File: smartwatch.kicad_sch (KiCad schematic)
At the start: 53 parts, among them IC1 W25N01GVZEIG, IC2 NORA-B120-00B, IC3 LM66200DRLR, J1 Charging_Pad-, J2 Charging_Pad+, J3 DS1020-09-15VBT1A, J4 Conn_01x04_Pin, Q1 2N7002, U1 MAX17048G+T10, U11 MCP73831T-2ACI/OT, U2 RV-3028-C7_32.768KHZ_1PPM-TA-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, U3 MAX30102, U4 TPS63001DRCR, U5 CAM-M8C-0, U6 AP7313-18SAG-7, U9 LIS2DE12, X2 9HT10-32.768KBZC-T

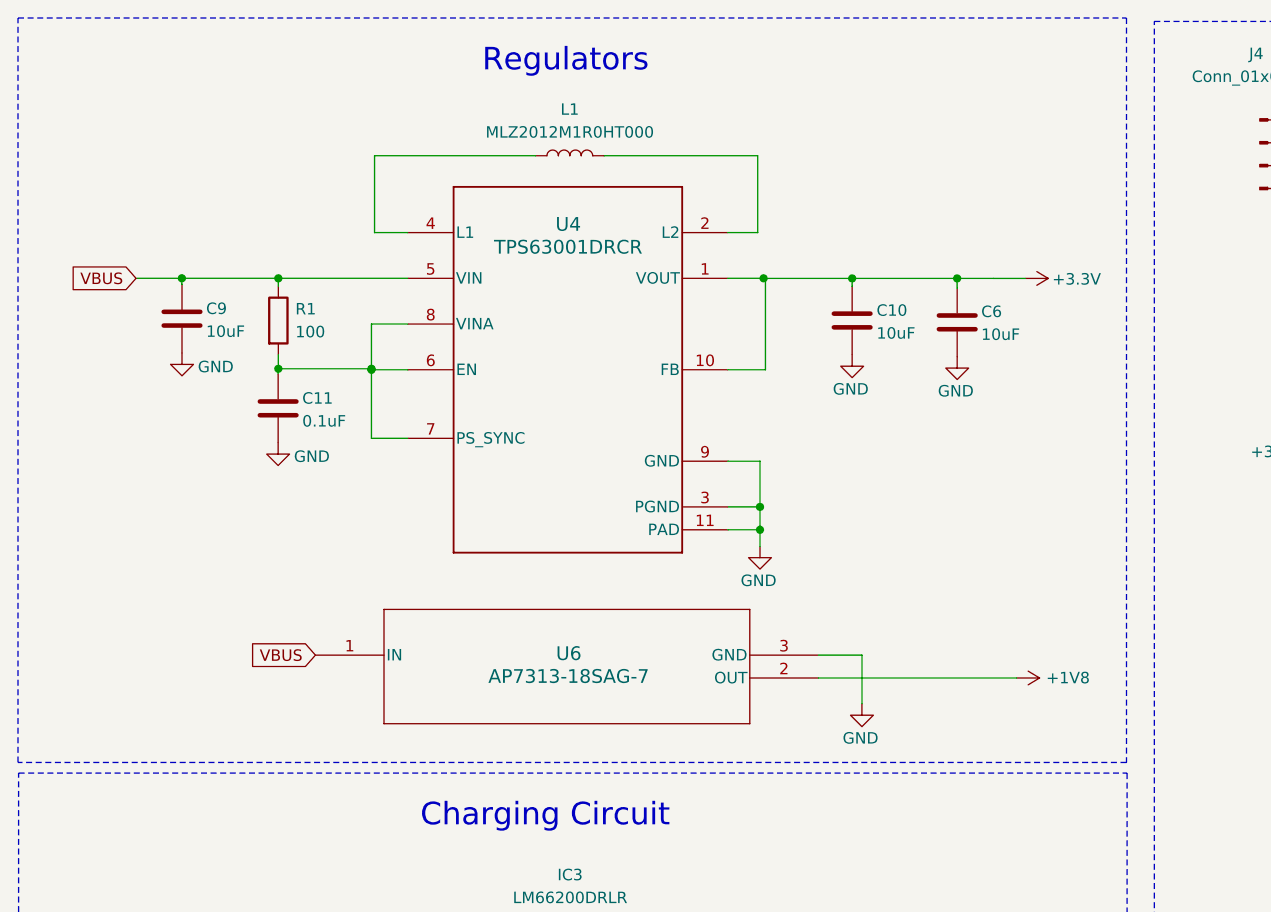
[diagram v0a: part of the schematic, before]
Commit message: update 1
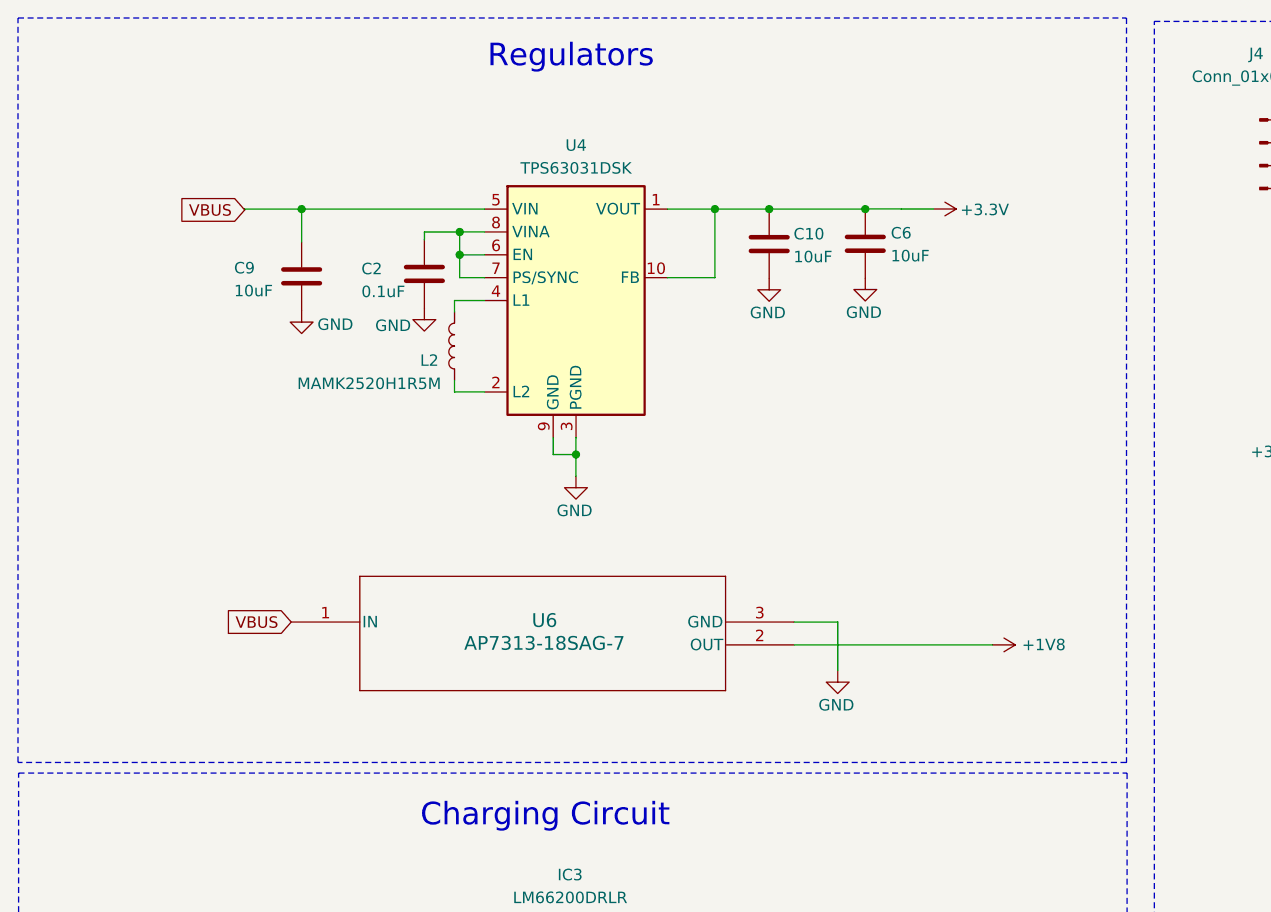
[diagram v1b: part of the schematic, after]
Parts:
- removed C11: 0.1uF, Capacitor_SMD:C_0402_1005Metric, symbol Device:C
- removed L1: MLZ2012M1R0HT000, Inductor_SMD:L_0805_2012Metric, symbol Device:L
- removed R1: 100, Resistor_SMD:R_0402_1005Metric, symbol Device:R
- removed U4: TPS63001DRCR, DRC0010J, symbol TPS63001DRCR:TPS63001DRCR
- added C2: 0.1uF, Capacitor_SMD:C_0402_1005Metric, symbol Device:C
- added L2: MAMK2520H1R5M, Inductor_SMD:L_1008_2520Metric, symbol Device:L
- added U4: TPS63031DSK, Package_SON:WSON-10-1EP_2.5x2.5mm_P0.5mm_EP1.2x2mm, symbol Regulator_Switching:TPS63031DSK
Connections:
- net +3.3V: now also U4.1 (VOUT), U4.10 (FB)
- net GND: now also C2.2, U4.11 (PGND), U4.3 (PGND), U4.9 (GND)
- net VBUS: now also U4.5 (VIN)
- new net: C2.1, U4.6 (EN), U4.7 (PS/SYNC), U4.8 (VINA)
- new net: L2.1, U4.2 (L2)
- new net: L2.2, U4.4 (L1)
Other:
- moved on the sheet: C10, C6, C9, U6
